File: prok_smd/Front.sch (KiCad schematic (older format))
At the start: 33 parts, among them CON1 microSD_Card, J12 Conn_01x05_Male, J15 Conn_01x02_Male, J16 Conn_01x02_Male, J17 Conn_01x02_Male, J18 Conn_01x02_Male, J5 TIME_CV, J6 CHANNEL_CV, J7 RESET_CV, J8 OUT, SW1 KS01BL

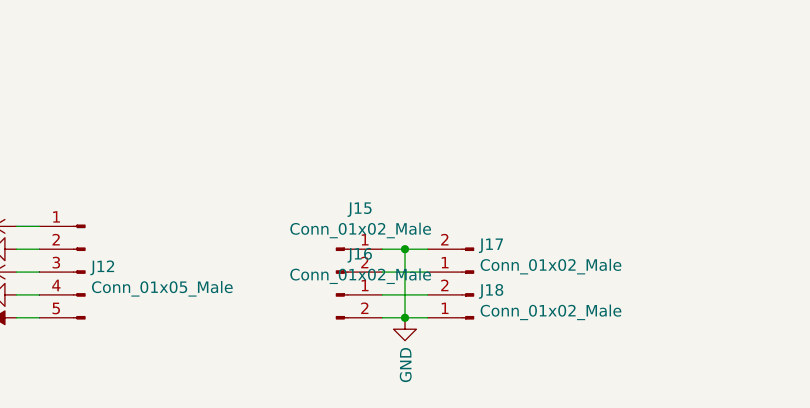
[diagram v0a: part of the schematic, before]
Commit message: :construction: first draft routing
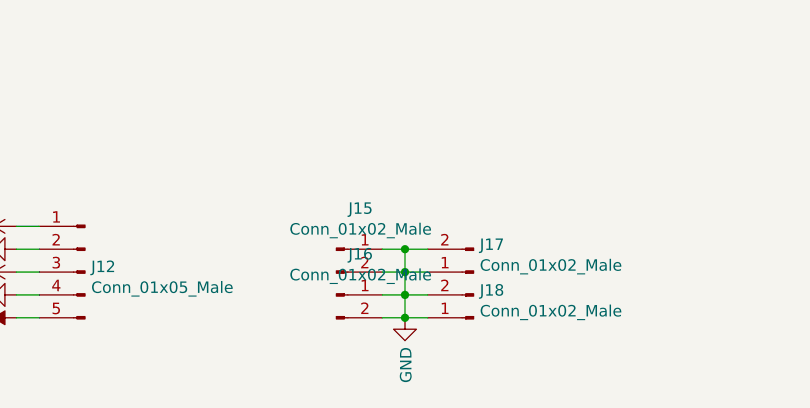
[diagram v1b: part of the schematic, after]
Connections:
- wire segments 64 -> 68
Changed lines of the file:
@@
 	4350 7250 4450 7250
-Wire Wire Line
-	4450 7150 4250 7150
-Wire Wire Line
-	4250 7050 4450 7050
 Wire Wire Line
 	4450 6950 4350 6950
 Wire Wire Line
-	4350 6950 4350 7250
+	4350 6950 4350 7050
 Connection ~ 4350 6950
 Wire Wire Line
@@
 	-1   0    0    1
 $EndComp
+Wire Wire Line
+	4250 7050 4350 7050
+Connection ~ 4350 7050
+Wire Wire Line
+	4350 7050 4350 7150
+Wire Wire Line
+	4350 7050 4450 7050
+Wire Wire Line
+	4250 7150 4350 7150
+Connection ~ 4350 7150
+Wire Wire Line
+	4350 7150 4350 7250
+Wire Wire Line
+	4350 7150 4450 7150
 $EndSCHEMATC
